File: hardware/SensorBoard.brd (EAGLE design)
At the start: 100.3 x 44.5 mm, 185 parts, among them IC1 SI7006-A10-IM, IC3 DWM1000, IC4 BMP280, IC5 FT232R, Q1 MC-306, T3 BC337, T4 BC337, U1 ESP-WROOM-32, U3 UM18533, X2 SMA-142-0711-821/826, X3 USB-MICRO-B-BOTTOM

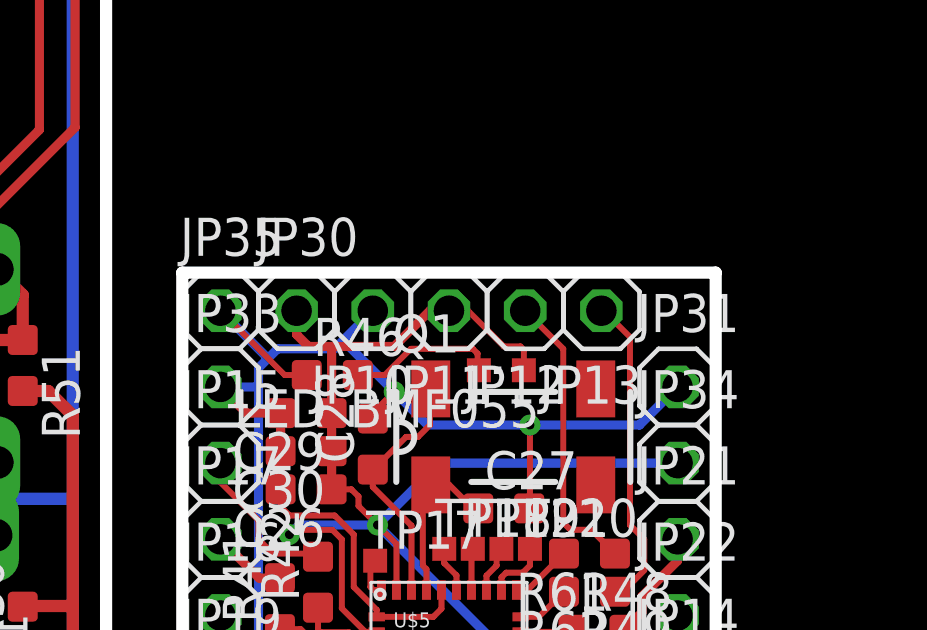
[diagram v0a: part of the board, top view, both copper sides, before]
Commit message: Cleaned hardware data.
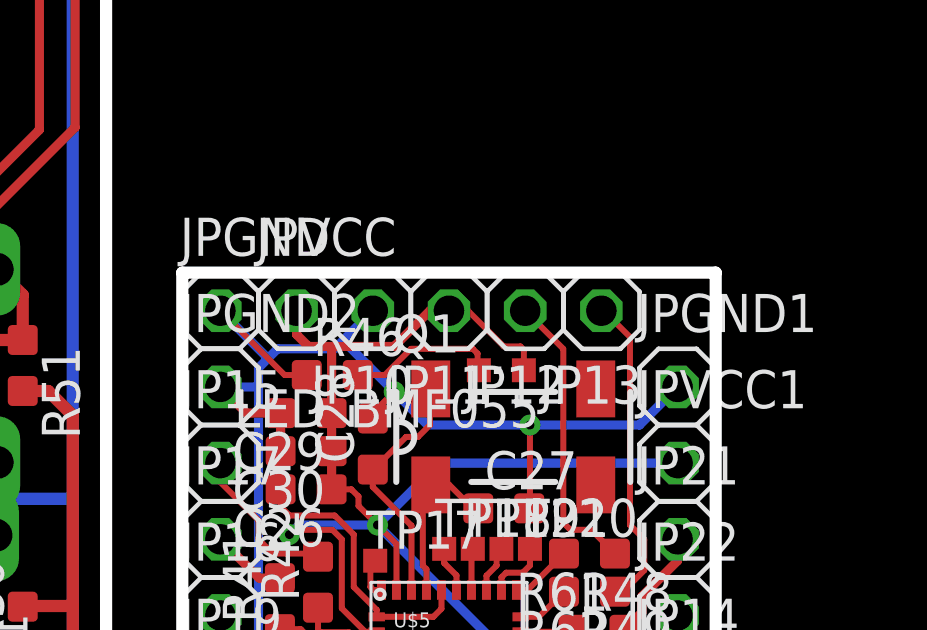
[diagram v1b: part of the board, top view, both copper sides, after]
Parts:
- renumbered JP30 to JPVCC, JP31 to JPGND1, JP33 to JPGND2, JP34 to JPVCC1, JP35 to JPGND
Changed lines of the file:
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@@
 <?xml version="1.0" encoding="utf-8"?>
 <!DOCTYPE eagle SYSTEM "eagle.dtd">
-<eagle version="7.5.0">
+<eagle version="6.5.0">
 <drawing>
 <settings>
@@
 <pass name="Default">
 <param name="RoutingGrid" value="50mil"/>
-<param name="AutoGrid" value="1"/>
-<param name="Efforts" value="0"/>
-<param name="TopRouterVariant" value="1"/>
 <param name="tpViaShape" value="round"/>
-<param name="PrefDir.1" value="a"/>
+<param name="PrefDir.1" value="|"/>
 <param name="PrefDir.2" value="0"/>
 <param name="PrefDir.3" value="0"/>
@@
 <param name="PrefDir.14" value="0"/>
 <param name="PrefDir.15" value="0"/>
-<param name="PrefDir.16" value="a"/>
+<param name="PrefDir.16" value="-"/>
 <param name="cfVia" value="8"/>
 <param name="cfNonPref" value="5"/>
@@
 <element name="JP27" library="pinhead" package="1X01" value="" x="52.705" y="34.925" rot="R270"/>
 <element name="JP28" library="pinhead" package="1X01" value="" x="52.705" y="32.385" rot="R270"/>
-<element name="JP30" library="pinhead" package="1X01" value="" x="86.36" y="19.685"/>
-<element name="JP31" library="pinhead" package="1X01" value="" x="99.06" y="17.145"/>
-<element name="JP33" library="pinhead" package="1X01" value="" x="83.82" y="17.145"/>
-<element name="JP34" library="pinhead" package="1X01" value="" x="99.06" y="14.605"/>
-<element name="JP35" library="pinhead" package="1X01" value="" x="83.82" y="19.685"/>
+<element name="JPVCC" library="pinhead" package="1X01" value="" x="86.36" y="19.685"/>
+<element name="JPGND1" library="pinhead" package="1X01" value="" x="99.06" y="17.145"/>
+<element name="JPGND2" library="pinhead" package="1X01" value="" x="83.82" y="17.145"/>
+<element name="JPVCC1" library="pinhead" package="1X01" value="" x="99.06" y="14.605"/>
+<element name="JPGND" library="pinhead" package="1X01" value="" x="83.82" y="19.685"/>
 </elements>
 <signals>
@@
 <wire x1="57.62625" y1="36.67125" x2="54.61" y2="33.655" width="0.2" layer="16"/>
 <wire x1="54.61" y1="33.655" x2="54.371875" y2="33.655" width="0.2" layer="16"/>
-<contactref element="JP30" pad="1"/>
-<contactref element="JP34" pad="1"/>
+<contactref element="JPVCC" pad="1"/>
+<contactref element="JPVCC1" pad="1"/>
 <wire x1="91.1225" y1="14.605" x2="89.05875" y2="12.54125" width="0.3048" layer="16"/>
 <wire x1="86.36" y1="18.89125" x2="86.36" y2="19.685" width="0.3048" layer="1"/>
@@
 <wire x1="57.864375" y1="26.273125" x2="58.89625" y2="27.305" width="0.3048" layer="16"/>
 <wire x1="58.89625" y1="27.305" x2="60.325" y2="27.305" width="0.3048" layer="16"/>
-<contactref element="JP31" pad="1"/>
-<contactref element="JP33" pad="1"/>
-<contactref element="JP35" pad="1"/>
+<contactref element="JPGND1" pad="1"/>
+<contactref element="JPGND2" pad="1"/>
+<contactref element="JPGND" pad="1"/>
 <wire x1="85.09" y1="17.145" x2="83.82" y2="17.145" width="0.3048" layer="16"/>
 <wire x1="88.9" y1="19.685" x2="87.9078125" y2="18.6928125" width="0.3048" layer="16"/>
